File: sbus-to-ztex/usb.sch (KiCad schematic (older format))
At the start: 13 parts, among them J4 USB_B_Micro, U5 SN65220, U7 TPS2051C

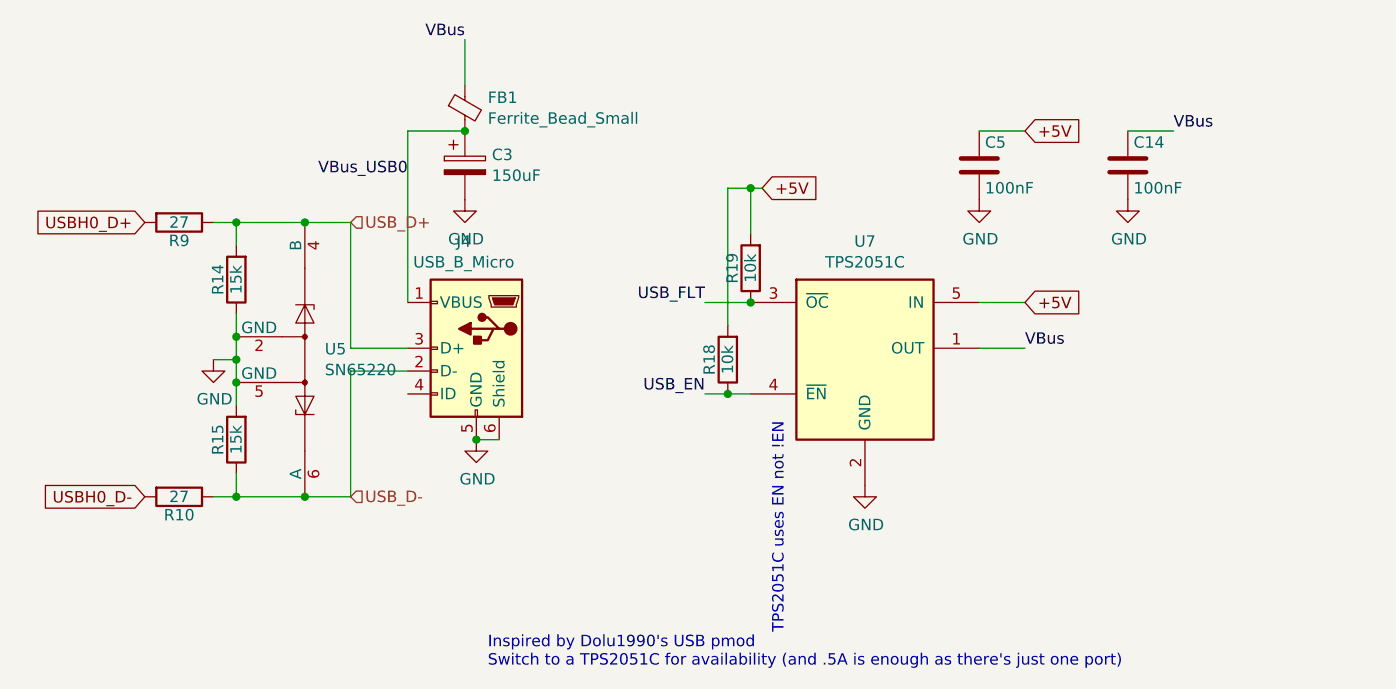
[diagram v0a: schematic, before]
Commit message: thinking about a V1.3
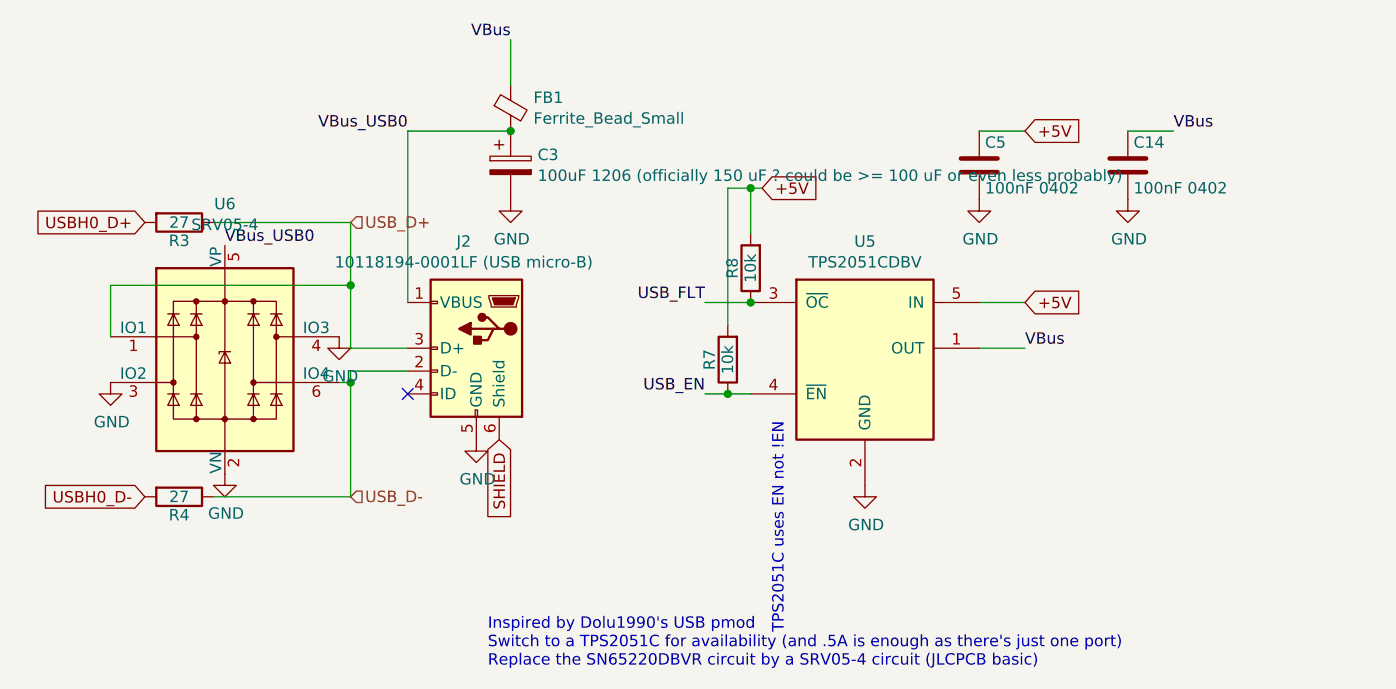
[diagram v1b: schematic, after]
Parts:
- removed R14, R15: 15k, Resistor_SMD:R_0603_1608Metric, symbol Device:R
- removed U5: SN65220, Package_TO_SOT_SMD:SOT-23-6, symbol Power_Protection:SN65220
- added U6: SRV05-4, Package_TO_SOT_SMD:SOT-23-6, symbol Power_Protection:SRV05-4
- C14, C5: value 100nF -> 100nF 0402; footprint Capacitor_SMD:C_0603_1608Metric -> Capacitor_SMD:C_0402_1005Metric; LCSC ? -> (none); MNF1_URL www.yageo.com -> (none); MPN CC0603KRX7R8BB104 -> CL05B104KO5NNNC; Mouser 603-CC603KRX7R8BB104 -> (none)
- C3: value 150uF -> 100uF 1206 (officially 150 uF ? could be >= 100 uF or even less probably); MPN GRM31CR60J157ME11L -> CL31A107MQHNNNE; MPN-ALT (none) -> GRM31CR60J157ME11L; MPN-ALT2 (none) -> JMK316ABJ107ML-T; URL (none) -> https://www.lcsc.com/product-detail/Multilayer-Ceramic-Capa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; URL-ALT (none) -> https://lcsc.com/product-detail/Multilayer-Ceramic-Capacito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; URL-ALT (mouser) (none) -> https://www.mouser.fr/ProductDetail/Murata-Electronics/GRM3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; URL-ALT2 (none) -> https://www.lcsc.com/product-detail/Multilayer-Ceramic-Capa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
- FB1: MPN PZ2012U221-2R0TF -> BLM21PG221SN1D; MPN-ALT2 (none) -> PZ2012U221-2R0TF; URL (none) -> https://www.lcsc.com/product-detail/Ferrite-Beads_Murata-El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; URL-ALT2 (none) -> https://www.lcsc.com/product-detail/Ferrite-Beads_Sunlord-P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
- J2: renamed from J4; value USB_B_Micro -> 10118194-0001LF (USB micro-B); footprint Connector_USB:USB_Micro-B_Molex-105017-0001 -> Connector_USB:USB_Micro-B_Amphenol_10118194_Horizontal; Description CONN RCPT USB2.0 MICRO B SMD R/A -> (none); Digi-Key_PN WM1399CT-ND -> (none); MPN 1050170001 -> 10118194-0001LF; Manufacturer Molex -> (none); URL https://eu.mouser.com/ProductDetail/Molex/105017-0001?qs=hl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 -> https://www.lcsc.com/product-detail/USB-Connectors_Amphenol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
- R3: renamed from R9; MPN-ALT ERJ-3EKF27R0V -> (none)
- R4: renamed from R10; MPN-ALT ERJ-3EKF27R0V -> (none)
- R7: renamed from R18; footprint Resistor_SMD:R_0603_1608Metric -> Resistor_SMD:R_0402_1005Metric; MPN 0603WAF1002T5E -> 0402WGF1002TCE
- R8: renamed from R19; footprint Resistor_SMD:R_0603_1608Metric -> Resistor_SMD:R_0402_1005Metric; MPN 0603WAF1002T5E -> 0402WGF1002TCE
- U5: renamed from U7; value TPS2051C -> TPS2051CDBV; URL https://www.mouser.fr/ProductDetail/Texas-Instruments/TPS20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 -> https://lcsc.com/product-detail/Power-Distribution-Switches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; URL (Mouser) (none) -> https://www.mouser.fr/ProductDetail/Texas-Instruments/TPS20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
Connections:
- net GND: now also U6.2 (VN), U6.3 (IO2), U6.4 (IO3); no longer J2.6 (Shield)
- net USB_D+: now also U6.1 (IO1)
- net USB_D-: now also U6.6 (IO4)
- net VBus_USB0: now also U6.5 (VP)
- new net SHIELD: J2.6 (Shield)
- no-connect marks 0 -> 1
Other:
- note added: "Inspired by Dolu1990's USB pmod\nSwitch to a TPS2051C for availability (and .5A is enough as there's just one port)\nReplace the SN65220DBVR circuit by a SRV05-4 circuit (JLCPCB basic)"
- note removed: "Inspired by Dolu1990's USB pmod\nSwitch to a TPS2051C for availability (and .5A is enough as there's just one port)\n"
- moved on the sheet: C3, FB1
